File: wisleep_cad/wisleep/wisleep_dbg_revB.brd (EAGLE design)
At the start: 20.3 x 15.2 mm, 3 parts

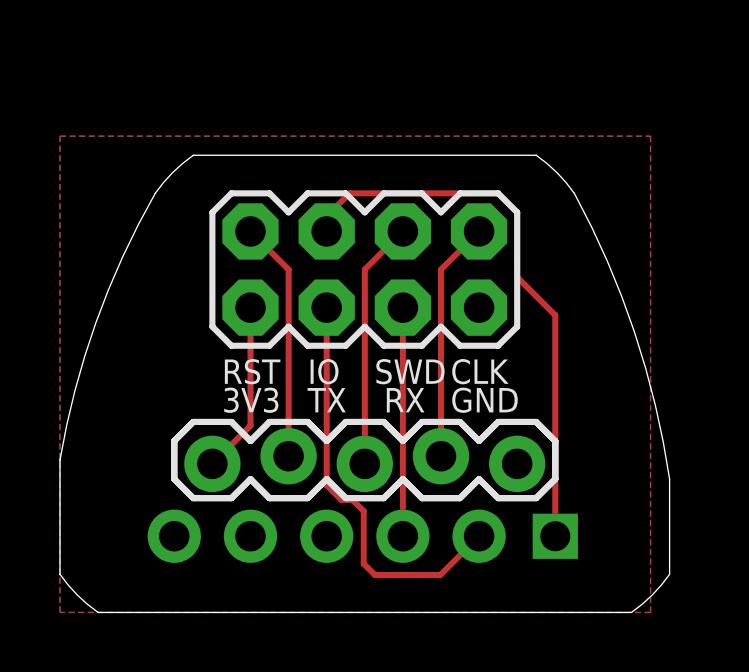
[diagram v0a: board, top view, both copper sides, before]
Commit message: cad: rev B to fab
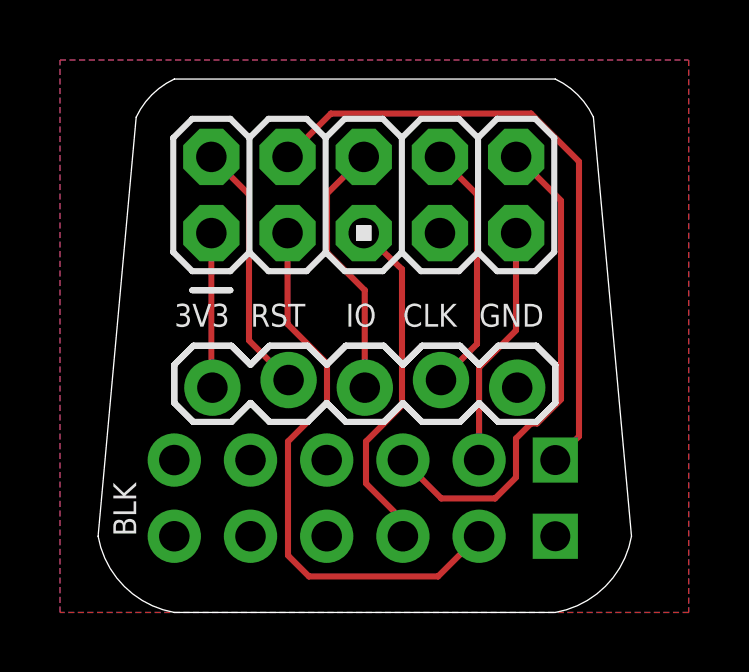
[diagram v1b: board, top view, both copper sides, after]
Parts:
- removed U$2: M04X2, SparkFun-Connectors:2X4
- added JP2: FTDI_DEVICE, SparkFun-Connectors:FTDI_DEVICE_SIDE
- added JP4: M05X2PTH, SparkFun-Connectors:AVR_ICSP
- moved JP3 2.54 mm to (15.2, 7.62)
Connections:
- new net WRX: JP2.P$3, JP4.10
- new net WTX: JP2.P$2, JP4.9
- net 3.3V: now also JP4.1; no longer U$2.1
- net DBG_IO: now also JP2.P$1, JP4.4; no longer JP1.P$1, U$2.4
- net GND: now also JP2.P$6, JP4.7; no longer U$2.7
- net RST: now also JP4.2; no longer U$2.2
- net SWCLK: now also JP4.8; no longer U$2.8
- net SWDIO: now also JP4.6; no longer U$2.6
- net USART_RX: now also JP4.5; no longer U$2.5
- net USART_TX: now also JP4.3; no longer U$2.3
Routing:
- net WRX: track 0.00 -> 16.7 mm
- net WTX: track 0.00 -> 8.08 mm
- net USART_TX: track 13.8 -> 19.0 mm
- net USART_RX: track 7.62 -> 11.7 mm
- net DBG_IO: track 18.8 -> 21.3 mm
- net 3.3V: track 5.73 -> 5.17 mm
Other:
- board size 20.3 x 15.2 mm -> 17.8 x 17.8 mm
- board text removed: "GRN"
- board text removed: "RX"
- board text removed: "SWD"
- board text removed: "TX"
